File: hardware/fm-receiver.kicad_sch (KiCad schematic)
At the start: 0 parts

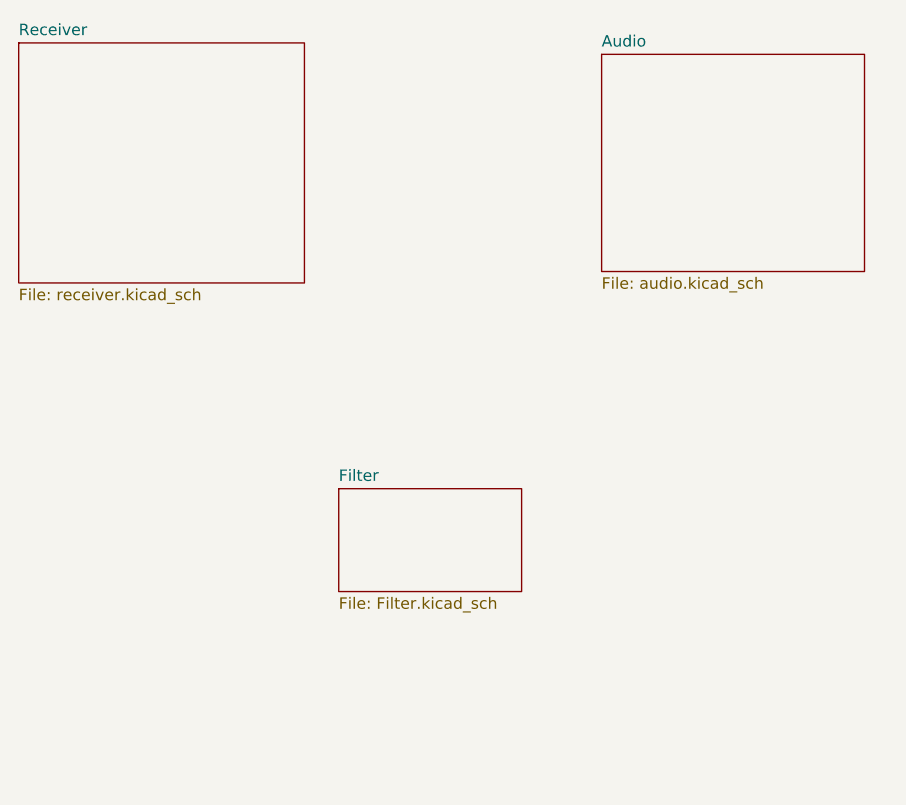
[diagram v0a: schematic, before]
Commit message: hardware: finishing schematics
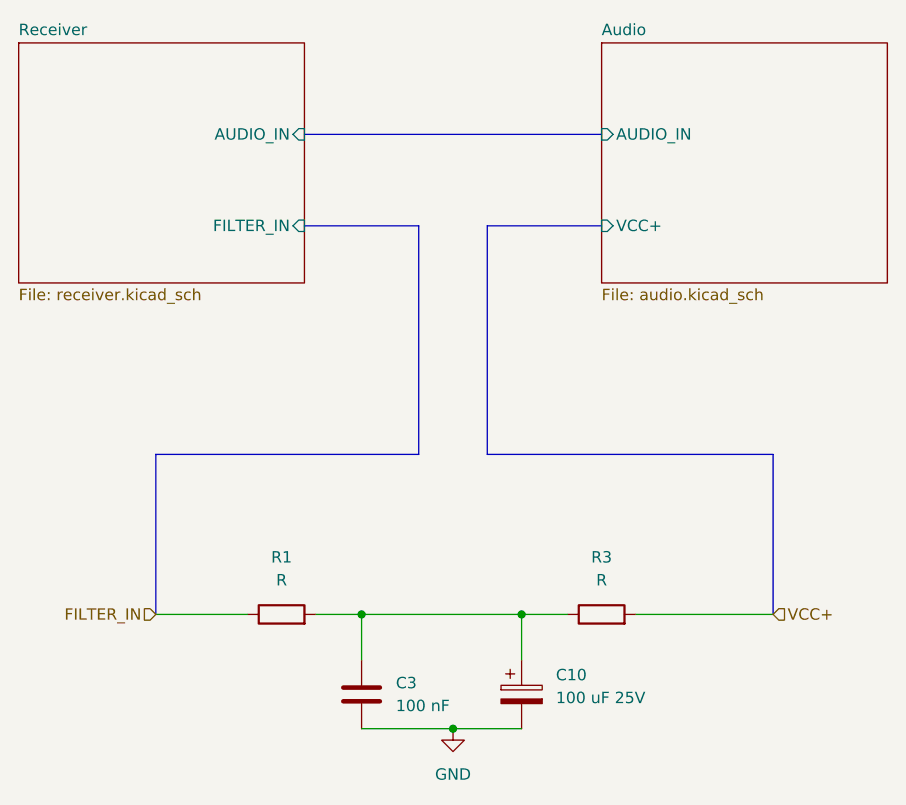
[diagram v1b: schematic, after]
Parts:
- added C10: 100 uF 25V, symbol Device:C_Polarized
- added C3: 100 nF, symbol Device:C
- added R1, R3: R, symbol Device:R
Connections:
- new net: C10.1, C3.1, R1.2, R3.1
- new net FILTER_IN: R1.1
- new net GND: C10.2, C3.2
- new net VCC+: R3.2
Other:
- removed sheet Filter
- sheet Audio ports: added AUDIO_IN, VCC+; removed none
- sheet Receiver ports: added AUDIO_IN, FILTER_IN; removed none

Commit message: hardware: starting layout
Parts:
- C10: footprint (none) -> Capacitor_THT:CP_Radial_D5.0mm_P2.50mm
- C3: footprint (none) -> Capacitor_THT:C_Disc_D4.3mm_W1.9mm_P5.00mm
- R1, R3: footprint (none) -> Resistor_THT:R_Axial_DIN0207_L6.3mm_D2.5mm_P10.16mm_Horizontal
